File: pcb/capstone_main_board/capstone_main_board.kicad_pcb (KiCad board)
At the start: 2 copper layers, 50 parts, among them J1 Vin, J10 MOSI, J11 SCLK, J12 NCS, J13 Vin, J14 Reserved_3, J15 Reserved_11, J16 Int1, J17 Int2, J18 SDO, J19 BAT, J2 VDD OS, J20 IO14, J21 IO13, J22 IO10, J23 IO8, J24 IO6, J25 RX0, J26 TX0, J27 D+, J28 D-, J29 100, J3 VDDA, J30 5V, J31 RESET, J32 Vin, J4 MFIO, J5 VDD FS, J6 V2, J7 V1, J8 Motion, J9 MISO, Q1 BSS138, Q2 BSS138, U1 OMGS3, U2 ADXL345, U3 TPS73219DBVT, U5 VREG_SOT23-5

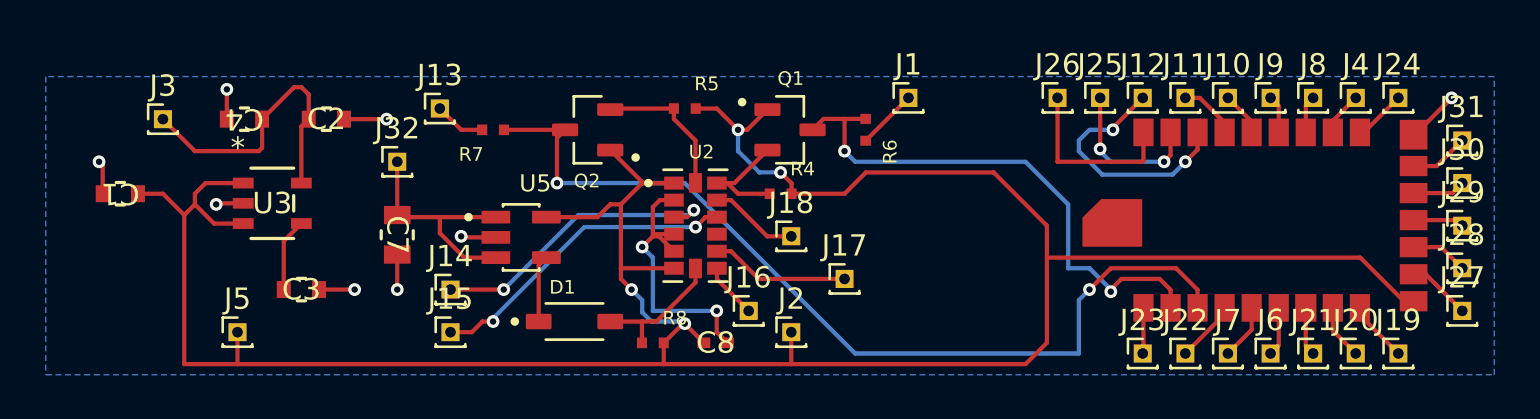
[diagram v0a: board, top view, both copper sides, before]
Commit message: sensor and mcu board nearly complete
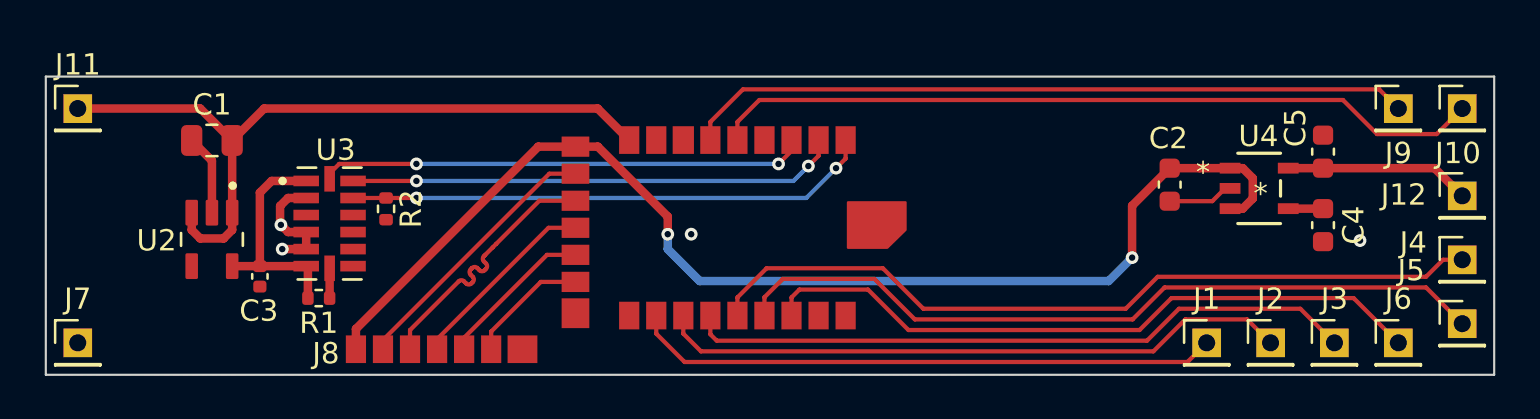
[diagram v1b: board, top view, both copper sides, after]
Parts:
- removed C7: 10µF, Library:CAP_CL21_SAM
- removed C8: 0.1uF, Library:CAP_CL05_SAM
- removed D1: 1N4148, Library:SOD3715X135N
- removed J13, J32: Vin, Connector_PinHeader_1.00mm:PinHeader_1x01_P1.00mm_Vertical
- removed J14: Reserved_3, Connector_PinHeader_1.00mm:PinHeader_1x01_P1.00mm_Vertical
- removed J15: Reserved_11, Connector_PinHeader_1.00mm:PinHeader_1x01_P1.00mm_Vertical
- removed J16: Int1, Connector_PinHeader_1.00mm:PinHeader_1x01_P1.00mm_Vertical
- removed J17: Int2, Connector_PinHeader_1.00mm:PinHeader_1x01_P1.00mm_Vertical
- removed J18: SDO, Connector_PinHeader_1.00mm:PinHeader_1x01_P1.00mm_Vertical
- removed J19: BAT, Connector_PinHeader_1.00mm:PinHeader_1x01_P1.00mm_Vertical
- removed J20: IO14, Connector_PinHeader_1.00mm:PinHeader_1x01_P1.00mm_Vertical
- removed J21: IO13, Connector_PinHeader_1.00mm:PinHeader_1x01_P1.00mm_Vertical
- removed J22: IO10, Connector_PinHeader_1.00mm:PinHeader_1x01_P1.00mm_Vertical
- removed J23: IO8, Connector_PinHeader_1.00mm:PinHeader_1x01_P1.00mm_Vertical
- removed J24: IO6, Connector_PinHeader_1.00mm:PinHeader_1x01_P1.00mm_Vertical
- removed J25: RX0, Connector_PinHeader_1.00mm:PinHeader_1x01_P1.00mm_Vertical
- removed J26: TX0, Connector_PinHeader_1.00mm:PinHeader_1x01_P1.00mm_Vertical
- removed J27: D+, Connector_PinHeader_1.00mm:PinHeader_1x01_P1.00mm_Vertical
- removed J28: D-, Connector_PinHeader_1.00mm:PinHeader_1x01_P1.00mm_Vertical
- removed J29: 100, Connector_PinHeader_1.00mm:PinHeader_1x01_P1.00mm_Vertical
- removed J30: 5V, Connector_PinHeader_1.00mm:PinHeader_1x01_P1.00mm_Vertical
- removed J31: RESET, Connector_PinHeader_1.00mm:PinHeader_1x01_P1.00mm_Vertical
- removed Q1, Q2: BSS138, Library:SOT95P240X111-3N
- removed R4, R5, R6, R7, R8: 10K, Library:RES_ERJ2RKF1002X
- removed U5: VREG_SOT23-5, Library:SOT95P285X140-5N
- added C5: 1uF, Capacitor_SMD:C_0603_1608Metric, F.Cu at (170.0, 56.5)
- added R1: 10K, Resistor_SMD:R_0402_1005Metric, F.Cu at (122.8, 63.4)
- added R2: 10k, Resistor_SMD:R_0402_1005Metric, F.Cu at (126.0, 59.2)
- added U4: TPS73219DBVT, Imported_FP:DBV5_TEX, F.Cu at (167.0, 58.3)
- C1: value 1uF -> 10uF; footprint Library:CAP_CL10_SAM -> Capacitor_SMD:C_0805_2012Metric
- C2, C4: footprint Library:CAP_CL10_SAM -> Capacitor_SMD:C_0603_1608Metric
- C3: value 1uF -> 0.1uF; footprint Library:CAP_CL10_SAM -> Capacitor_SMD:C_0402_1005Metric
- J1: value Vin -> MFIO; footprint Connector_PinHeader_1.00mm:PinHeader_1x01_P1.00mm_Vertical -> Connector_PinHeader_2.00mm:PinHeader_1x01_P2.00mm_Vertical
- J10: value MOSI -> FORCE_V1; footprint Connector_PinHeader_1.00mm:PinHeader_1x01_P1.00mm_Vertical -> Connector_PinHeader_2.00mm:PinHeader_1x01_P2.00mm_Vertical
- J11: value SCLK -> VBAT+; footprint Connector_PinHeader_1.00mm:PinHeader_1x01_P1.00mm_Vertical -> Connector_PinHeader_2.00mm:PinHeader_1x01_P2.00mm_Vertical
- J12: value NCS -> VDDA; footprint Connector_PinHeader_1.00mm:PinHeader_1x01_P1.00mm_Vertical -> Connector_PinHeader_2.00mm:PinHeader_1x01_P2.00mm_Vertical
- J2: value VDD OS -> Motion; footprint Connector_PinHeader_1.00mm:PinHeader_1x01_P1.00mm_Vertical -> Connector_PinHeader_2.00mm:PinHeader_1x01_P2.00mm_Vertical
- J3: value VDDA -> MISO; footprint Connector_PinHeader_1.00mm:PinHeader_1x01_P1.00mm_Vertical -> Connector_PinHeader_2.00mm:PinHeader_1x01_P2.00mm_Vertical
- J4: value MFIO -> MOSI; footprint Connector_PinHeader_1.00mm:PinHeader_1x01_P1.00mm_Vertical -> Connector_PinHeader_2.00mm:PinHeader_1x01_P2.00mm_Vertical
- J5: value VDD FS -> SCLK; footprint Connector_PinHeader_1.00mm:PinHeader_1x01_P1.00mm_Vertical -> Connector_PinHeader_2.00mm:PinHeader_1x01_P2.00mm_Vertical
- J6: value V2 -> NCS; footprint Connector_PinHeader_1.00mm:PinHeader_1x01_P1.00mm_Vertical -> Connector_PinHeader_2.00mm:PinHeader_1x01_P2.00mm_Vertical
- J7: value V1 -> VBAT-; footprint Connector_PinHeader_1.00mm:PinHeader_1x01_P1.00mm_Vertical -> Connector_PinHeader_2.00mm:PinHeader_1x01_P2.00mm_Vertical
- J8: value Motion -> Conn_01x07_Pin; footprint Connector_PinHeader_1.00mm:PinHeader_1x01_P1.00mm_Vertical -> Custom_FP:OMGS3_programming_pins
- J9: value MISO -> FORCE_V2; footprint Connector_PinHeader_1.00mm:PinHeader_1x01_P1.00mm_Vertical -> Connector_PinHeader_2.00mm:PinHeader_1x01_P2.00mm_Vertical
- U1: footprint Library:OMGS3 -> Imported_FP:OMGS3
- U2: value ADXL345 -> VREG_SOT23-5; footprint Library:PQFN80P500X300X100-14N -> Imported_FP:SOT95P280X145-5N
- U3: value TPS73219DBVT -> ADXL345; footprint Library:DBV5_TEX -> Imported_FP:PQFN80P500X300X100-14N
- moved J5 57.5 mm to (176.5, 64.6)
- moved J3 56.0 mm to (170.5, 65.5)
- moved J7 54.0 mm to (111.5, 65.5)
- moved J11 52.0 mm to (111.5, 54.5)
- moved C4 50.9 mm to (170.0, 60.0), turned to -90 degrees
- moved J8 42.8 mm to (128.4, 65.8), turned to 90 degrees
- moved U1 42.4 mm to (134.0, 65.1), turned to 0 degrees
- moved C2 39.7 mm to (162.8, 58.1), turned to -90 degrees
- moved U2 22.7 mm to (117.8, 60.6), turned to -90 degrees
- moved J2 22.5 mm to (167.5, 65.5)
- moved J1 18.1 mm to (164.5, 65.5)
- moved J12 15.7 mm to (176.5, 58.6)
- moved J10 11.0 mm to (176.5, 54.5)
- moved J4 9.10 mm to (176.5, 61.6)
- moved J6 6.02 mm to (173.5, 65.5)
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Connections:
- C1 pad 1: Net-(J2-Pin_1) -> GND
- C1 pad 2: GND -> VBAT+
- C2 pad 1: Net-(J3-Pin_1) -> +3.3V
- C3 pad 1: Net-(U3-NR/FB) -> GND
- C3 pad 2: GND -> ACCEL_VIN
- C4 pad 1: Net-(J3-Pin_1) -> Net-(U4-NR/FB)
- J11 pad 1: Net-(J11-Pin_1) -> VBAT+
- J5 pad 1: Net-(J2-Pin_1) -> Net-(J5-Pin_1)
- J7 pad 1: Net-(J7-Pin_1) -> GND
- J8 pad 1: Net-(J8-Pin_1) -> GND
- U1 pad 1: Net-(J26-Pin_1) -> unconnected-(U1-TX0-Pad1)
- U1 pad 11: Net-(J31-Pin_1) -> Net-(J8-Pin_2)
- U1 pad 12: Net-(J30-Pin_1) -> Net-(J8-Pin_3)
- U1 pad 13: Net-(J29-Pin_1) -> Net-(J8-Pin_4)
- U1 pad 14: Net-(J28-Pin_1) -> Net-(J8-Pin_5)
- U1 pad 15: Net-(J27-Pin_1) -> Net-(J8-Pin_6)
- U1 pad 16: Net-(J2-Pin_1) -> +3.3V
- U1 pad 17: Net-(J19-Pin_1) -> VBAT+
- U1 pad 18: Net-(J20-Pin_1) -> unconnected-(U1-IO14-Pad18)
- U1 pad 19: Net-(J21-Pin_1) -> unconnected-(U1-IO13-Pad19)
- U1 pad 2: Net-(J25-Pin_1) -> unconnected-(U1-RX0-Pad2)
- U1 pad 20: Net-(J6-Pin_1) -> Net-(J9-Pin_1)
- U1 pad 21: Net-(J7-Pin_1) -> Net-(J10-Pin_1)
- U1 pad 22: Net-(J22-Pin_1) -> unconnected-(U1-IO10-Pad22)
- U1 pad 25: Net-(J23-Pin_1) -> /SDO/ADDR
- U1 pad 3: Net-(J12-Pin_1) -> Net-(J6-Pin_1)
- U1 pad 4: Net-(J11-Pin_1) -> Net-(J5-Pin_1)
- U1 pad 5: Net-(J10-Pin_1) -> Net-(J4-Pin_1)
- U1 pad 6: Net-(J9-Pin_1) -> Net-(J3-Pin_1)
- U1 pad 7: Net-(J8-Pin_1) -> Net-(J2-Pin_1)
- U1 pad 8: Net-(J4-Pin_1) -> Net-(J1-Pin_1)
- U1 pad 9: Net-(J24-Pin_1) -> unconnected-(U1-EN-Pad9)
- U2 pad 1: Net-(J2-Pin_1) -> VBAT+
- U2 pad 2: Net-(C8-Pad2) -> GND
- U2 pad 3: Net-(J14-Pin_1) -> VBAT+
- U2 pad 4: Net-(C8-Pad2) -> unconnected-(U2-P4-Pad4)
- U2 pad 5: Net-(C8-Pad2) -> ACCEL_VIN
- U3 pad 1: Net-(J2-Pin_1) -> ACCEL_VIN
- U3 pad 3: Net-(J2-Pin_1) -> unconnected-(U3-RESERVED_3-Pad3)
- U3 pad 4: Net-(U3-NR/FB) -> GND
- U3 pad 5: Net-(J3-Pin_1) -> GND
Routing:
- net Net-(J2-Pin_1): track 129.9 -> 29.8 mm, vias 4 -> 0
- net +3.3V: track 0.00 -> 56.1 mm, vias 0 -> 2
- net Net-(J5-Pin_1): track 0.00 -> 36.1 mm
- net Net-(J4-Pin_1): track 2.07 -> 37.6 mm
- net VBAT+: track 0.00 -> 35.0 mm
- net Net-(J10-Pin_1): track 2.08 -> 36.5 mm
- net Net-(J9-Pin_1): track 1.78 -> 34.2 mm
- net Net-(J6-Pin_1): track 2.30 -> 31.8 mm
- net Net-(J1-Pin_1): track 2.85 -> 27.6 mm
- net /SDO/ADDR: track 0.00 -> 24.8 mm, vias 0 -> 2
- net /SCL: track 43.3 -> 22.9 mm
- net Net-(J3-Pin_1): track 13.9 -> 31.6 mm
- net Net-(J15-Pin_1): track 14.8 -> 0.00 mm, vias 2 -> 0
- net Net-(J14-Pin_1): track 14.0 -> 0.00 mm, vias 2 -> 0
- net Net-(C8-Pad2): track 13.4 -> 0.00 mm, vias 2 -> 0
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- added copper zone on F.Cu, net GND
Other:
- board outline added: 68 x 14 mm
